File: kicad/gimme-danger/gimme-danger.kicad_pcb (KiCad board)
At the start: 4 copper layers, 48 x 42 mm, 94 parts, among them J3 Screw_Terminal_01x06, Q1 AO3400A, Q2 AO3400A, Q3 AO3400A, Q4 AO3400A, U1 ESP32-S3-WROOM-1, U11 DDTC143EUA, U2 TYPE-C-31-M-12, U3 TPD4E1U06DCKR, U4 DC-84, U5 SKRKAEE020, U7 SKRKAEE020, U8 TPS54302, U9 INA219AIDR

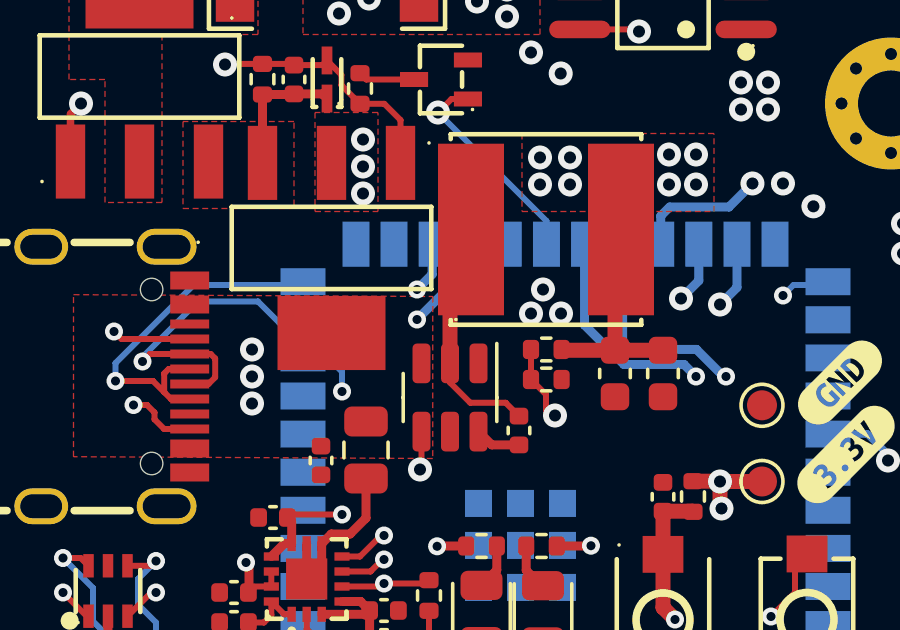
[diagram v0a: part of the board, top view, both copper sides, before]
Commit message: v0.0.2a fabrication
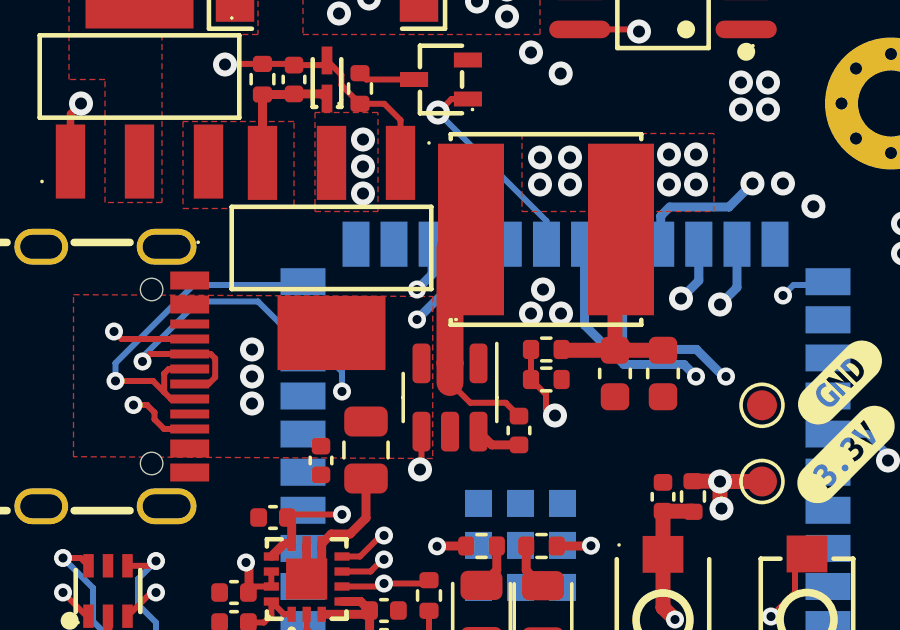
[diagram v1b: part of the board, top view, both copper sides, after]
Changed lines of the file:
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@@
     (property "Sheetfile" "gimme-danger.kicad_sch")
     (property "Sheetname" "")
+    (property "dnp" "")
+    (property "exclude_from_bom" "")
     (property "ki_description" "Mounting Hole with connection")
     (property "ki_keywords" "mounting hole")
     (zone_connect 2)
-    (attr exclude_from_pos_files)
+    (attr exclude_from_pos_files exclude_from_bom)
     (fp_text reference "H1" (at 0 -3.2) (layer "F.SilkS") hide
         (effects (font (size 1 1) (thickness 0.15)))
@@
       (net 25 "GND") (pinfunction "GND") (pintype "power_in") (zone_connect 2))
     (pad "2" smd roundrect (at -1.1375 0 270) (size 1.325 0.6) (layers "F.Cu" "F.Paste" "F.Mask") (roundrect_rratio 0.25)
-      (net 49 "Net-(U8-SW)") (pinfunction "SW") (pintype "power_out"))
+      (net 49 "Net-(U8-SW)") (pinfunction "SW") (pintype "power_out") (zone_connect 2))
     (pad "3" smd roundrect (at -1.1375 0.95 270) (size 1.325 0.6) (layers "F.Cu" "F.Paste" "F.Mask") (roundrect_rratio 0.25)
       (net 27 "VBUS") (pinfunction "VIN") (pintype "power_in") (zone_connect 2))
@@
     (property "Sheetfile" "gimme-danger.kicad_sch")
     (property "Sheetname" "")
+    (property "dnp" "")
+    (property "exclude_from_bom" "")
     (property "ki_description" "Mounting Hole with connection")
     (property "ki_keywords" "mounting hole")
     (zone_connect 2)
-    (attr exclude_from_pos_files)
+    (attr exclude_from_pos_files exclude_from_bom)
     (fp_text reference "H2" (at 0 -3.2) (layer "F.SilkS") hide
         (effects (font (size 1 1) (thickness 0.15)))
@@
     (property "Sheetfile" "gimme-danger.kicad_sch")
     (property "Sheetname" "")
+    (property "dnp" "")
+    (property "exclude_from_bom" "")
     (property "ki_description" "Mounting Hole with connection")
     (property "ki_keywords" "mounting hole")
     (zone_connect 2)
-    (attr exclude_from_pos_files)
+    (attr exclude_from_pos_files exclude_from_bom)
     (fp_text reference "H3" (at 0 -3.2) (layer "F.SilkS") hide
         (effects (font (size 1 1) (thickness 0.15)))
@@
     (property "Sheetfile" "gimme-danger.kicad_sch")
     (property "Sheetname" "")
+    (property "dnp" "")
+    (property "exclude_from_bom" "")
     (property "ki_keywords" "C718040")
     (zone_connect 2)
-    (attr through_hole)
+    (attr through_hole exclude_from_bom)
     (fp_text reference "U4" (at -2.25 -5.751054 90) (layer "F.SilkS") hide
         (effects (font (size 1 1) (thickness 0.15)))
@@
   (segment (start 75.1 107.1) (end 74.5 107.7) (width 0.5) (layer "F.Cu") (net 49))
   (segment (start 76.355 112.875) (end 75.175 112.875) (width 0.2) (layer "F.Cu") (net 49))
-  (segment (start 74.5 112.2) (end 74.5 111.5625) (width 0.2) (layer "F.Cu") (net 49))
+  (segment (start 74.5 112.2) (end 74.5 111.5625) (width 0.9) (layer "F.Cu") (net 49))
   (segment (start 75.175 112.875) (end 74.5 112.2) (width 0.2) (layer "F.Cu") (net 49))
-  (segment (start 74.5 107.7) (end 74.5 111.5625) (width 0.5) (layer "F.Cu") (net 49))
+  (segment (start 74.5 107.7) (end 74.5 111.5625) (width 0.9) (layer "F.Cu") (net 49))
   (segment (start 76.8 113.32) (end 76.355 112.875) (width 0.2) (layer "F.Cu") (net 49))
   (segment (start 75.9 107.1) (end 74.5 108.5) (width 0.5) (layer "F.Cu") (net 49))
